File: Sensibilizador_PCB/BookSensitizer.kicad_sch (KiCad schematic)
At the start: 27 parts, among them U1 LM5104M, U2 LM5104M

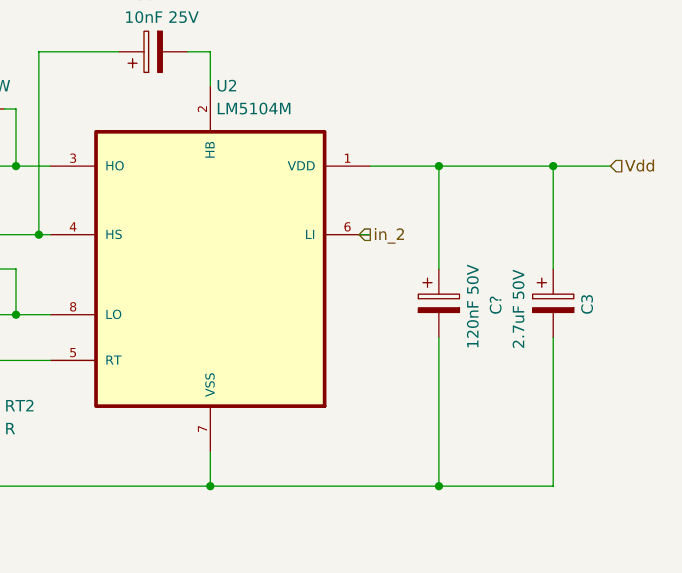
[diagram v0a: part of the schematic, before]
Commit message: pequeño cambio
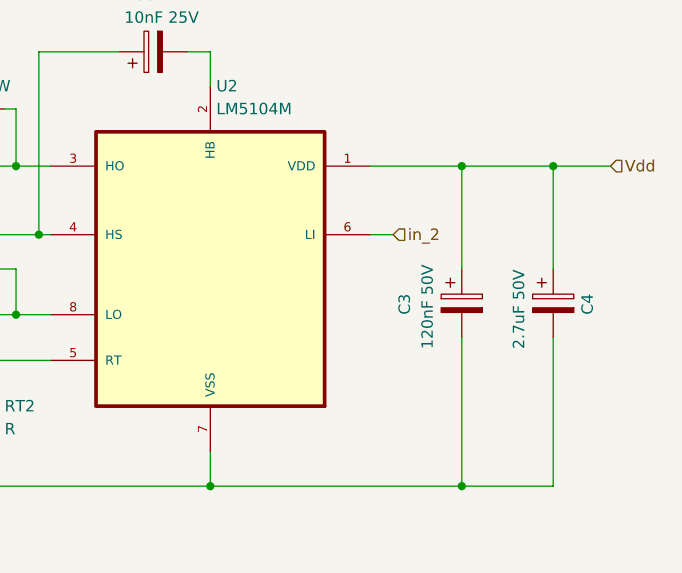
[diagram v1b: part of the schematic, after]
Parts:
- gave numbers to parts that had none: 1
- renumbered C3 to C4
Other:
- moved on the sheet: C3
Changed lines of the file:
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@@
   (junction (at 100.33 105.41) (diameter 0) (color 0 0 0 0)
   )
-  (junction (at 245.11 88.9) (diameter 0) (color 0 0 0 0)
-  )
   (junction (at 166.37 124.46) (diameter 0) (color 0 0 0 0)
   )
   (junction (at 44.45 88.9) (diameter 0) (color 0 0 0 0)
   )
-  (junction (at 245.11 124.46) (diameter 0) (color 0 0 0 0)
-  )
   (junction (at 200.66 96.52) (diameter 0) (color 0 0 0 0)
   )
@@
   (junction (at 97.79 96.52) (diameter 0) (color 0 0 0 0)
   )
+  (junction (at 247.65 124.46) (diameter 0) (color 0 0 0 0)
+  )
   (junction (at 100.33 88.9) (diameter 0) (color 0 0 0 0)
   )
+  (junction (at 247.65 88.9) (diameter 0) (color 0 0 0 0)
+  )
   (junction (at 194.31 124.46) (diameter 0) (color 0 0 0 0)
   )
@@
     (stroke (width 0) (type default) (color 0 0 0 0))
   )
+  (wire (pts (xy 247.65 88.9) (xy 257.81 88.9))
+    (stroke (width 0) (type default) (color 0 0 0 0))
+  )
   (wire (pts (xy 101.6 124.46) (xy 129.54 124.46))
     (stroke (width 0) (type default) (color 0 0 0 0))
@@
     (stroke (width 0) (type default) (color 0 0 0 0))
   )
-  (wire (pts (xy 245.11 107.95) (xy 245.11 124.46))
+  (wire (pts (xy 247.65 107.95) (xy 247.65 124.46))
     (stroke (width 0) (type default) (color 0 0 0 0))
   )
@@
     (stroke (width 0) (type default) (color 0 0 0 0))
   )
-  (wire (pts (xy 245.11 88.9) (xy 245.11 100.33))
+  (wire (pts (xy 247.65 88.9) (xy 247.65 100.33))
     (stroke (width 0) (type default) (color 0 0 0 0))
   )
@@
     (stroke (width 0) (type default) (color 0 0 0 0))
   )
-  (wire (pts (xy 245.11 88.9) (xy 257.81 88.9))
+  (wire (pts (xy 237.49 88.9) (xy 247.65 88.9))
     (stroke (width 0) (type default) (color 0 0 0 0))
   )
@@
     (stroke (width 0) (type default) (color 0 0 0 0))
   )
-  (wire (pts (xy 219.71 124.46) (xy 245.11 124.46))
+  (wire (pts (xy 219.71 124.46) (xy 247.65 124.46))
     (stroke (width 0) (type default) (color 0 0 0 0))
   )
@@
     (stroke (width 0) (type default) (color 0 0 0 0))
   )
+  (wire (pts (xy 237.49 96.52) (xy 240.03 96.52))
+    (stroke (width 0) (type default) (color 0 0 0 0))
+  )
   (wire (pts (xy 185.42 100.33) (xy 187.96 100.33))
     (stroke (width 0) (type default) (color 0 0 0 0))
   )
-  (wire (pts (xy 237.49 96.52) (xy 236.22 96.52))
-    (stroke (width 0) (type default) (color 0 0 0 0))
-  )
   (wire (pts (xy 119.38 82.55) (xy 119.38 88.9))
     (stroke (width 0) (type default) (color 0 0 0 0))
   )
-  (wire (pts (xy 237.49 88.9) (xy 245.11 88.9))
-    (stroke (width 0) (type default) (color 0 0 0 0))
-  )
   (wire (pts (xy 185.42 105.41) (xy 198.12 105.41))
     (stroke (width 0) (type default) (color 0 0 0 0))
   )
+  (wire (pts (xy 247.65 124.46) (xy 257.81 124.46))
+    (stroke (width 0) (type default) (color 0 0 0 0))
+  )
   (wire (pts (xy 180.34 88.9) (xy 176.53 88.9))
     (stroke (width 0) (type default) (color 0 0 0 0))
@@
   )
   (wire (pts (xy 118.11 82.55) (xy 119.38 82.55))
-    (stroke (width 0) (type default) (color 0 0 0 0))
-  )
-  (wire (pts (xy 245.11 124.46) (xy 257.81 124.46))
     (stroke (width 0) (type default) (color 0 0 0 0))
   )
@@
     (effects (font (size 1.27 1.27)) (justify left))
   )
-  (hierarchical_label "in_2" (shape input) (at 236.22 96.52 0)
+  (hierarchical_label "in_2" (shape input) (at 240.03 96.52 0)
     (effects (font (size 1.27 1.27)) (justify left))
   )
@@
   (symbol (lib_id "Device:C_Polarized") (at 257.81 104.14 0) (unit 1)
     (in_bom yes) (on_board yes)
-    (property "Reference" "C3" (id 0) (at 261.62 105.41 90)
+    (property "Reference" "C4" (id 0) (at 261.62 105.41 90)
       (effects (font (size 1.27 1.27)) (justify left))
     )
@@
     (pin "2")
   )
-  (symbol (lib_id "Device:C_Polarized") (at 245.11 104.14 0) (unit 1)
-    (in_bom yes) (on_board yes)
-    (property "Reference" "C?" (id 0) (at 251.46 105.41 90)
-      (effects (font (size 1.27 1.27)) (justify left))
-    )
-    (property "Value" "120nF 50V" (id 1) (at 248.92 109.22 90)
-      (effects (font (size 1.27 1.27)) (justify left))
-    )
-    (property "Footprint" "" (id 2) (at 246.0752 107.95 0)
-      (effects (font (size 1.27 1.27)) hide)
-    )
-    (property "Datasheet" "~" (id 3) (at 245.11 104.14 0)
+  (symbol (lib_id "Device:C_Polarized") (at 247.65 104.14 0) (unit 1)
+    (in_bom yes) (on_board yes)
+    (property "Reference" "C3" (id 0) (at 241.3 105.41 90)
+      (effects (font (size 1.27 1.27)) (justify left))
+    )
+    (property "Value" "120nF 50V" (id 1) (at 243.84 109.22 90)
+      (effects (font (size 1.27 1.27)) (justify left))
+    )
+    (property "Footprint" "" (id 2) (at 248.6152 107.95 0)
+      (effects (font (size 1.27 1.27)) hide)
+    )
+    (property "Datasheet" "~" (id 3) (at 247.65 104.14 0)
       (effects (font (size 1.27 1.27)) hide)
     )
@@
       (reference "C2") (unit 1) (value "120nF 50V") (footprint "")
     )
+    (path "/48faf4b4-702a-461e-beb4-48d0c1e72cc8"
+      (reference "C3") (unit 1) (value "120nF 50V") (footprint "")
+    )
     (path "/465bacb8-855b-413b-b25f-0e807e6db853"
-      (reference "C3") (unit 1) (value "2.7uF 50V") (footprint "")
-    )
-    (path "/48faf4b4-702a-461e-beb4-48d0c1e72cc8"
-      (reference "C?") (unit 1) (value "120nF 50V") (footprint "")
+      (reference "C4") (unit 1) (value "2.7uF 50V") (footprint "")
     )
     (path "/67aed173-e197-46ac-a867-f62a7f385d0c"
